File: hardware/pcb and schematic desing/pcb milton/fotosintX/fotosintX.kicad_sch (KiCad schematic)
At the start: 15 parts, among them J4 TB_1X2, J5 TB_1X2, Q1 PN2222A, U1 ESP32_DEVKITC, U2 L7805

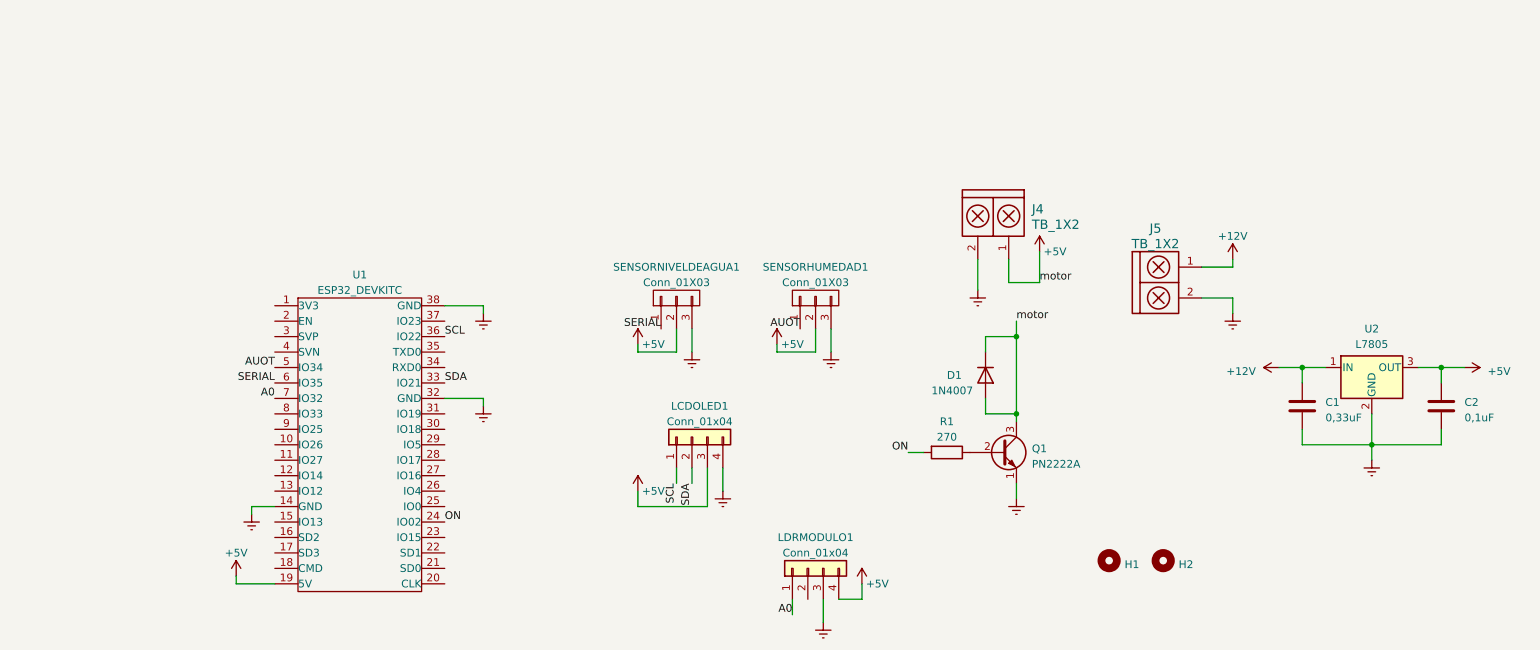
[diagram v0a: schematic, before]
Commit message: arregle el schematic
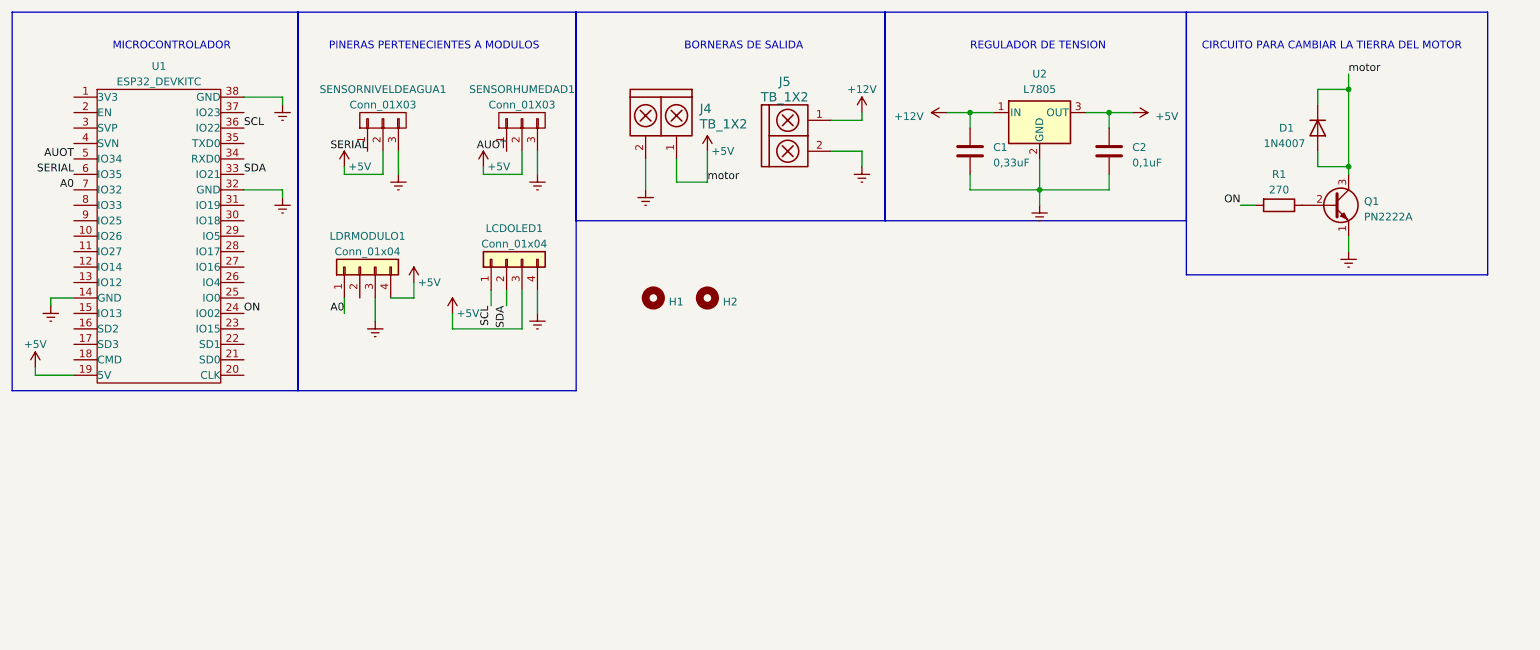
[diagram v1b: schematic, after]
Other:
- note added: "BORNERAS DE SALIDA"
- note added: "CIRCUITO PARA CAMBIAR LA TIERRA DEL MOTOR"
- note added: "MICROCONTROLADOR"
- note added: "PINERAS PERTENECIENTES A MODULOS"
- note added: "REGULADOR DE TENSION"
- moved on the sheet: C1, C2, D1, H1, H2, J4, J5, LCDOLED1, LDRMODULO1, Q1, R1, SENSORHUMEDAD1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
